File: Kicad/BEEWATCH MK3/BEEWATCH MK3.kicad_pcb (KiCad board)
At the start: 2 copper layers, 40 x 40 mm, 103 parts, among them J1 USB_C_Receptacle_USB2.0, J3 Conn_02x06_Odd_Even, Q1 2N7002, Q2 2N7002, Q3 DMP1045U-7, Q4 BSS138, Q5 BSS138, Q6 BSS138, Q7 BSS138, SW1 TK-074-4, SW2 TK-074-4, U1 ESP32-S3, U3 MPU-6050, U4 MCP73832-2-OT, U5 ME6217C33M5G, U6 LTC3549EDCB#TRMPBF, U7 RYS8830, U8 S-1206B18-M3T1G, Y1 40MHz, Y2 32.768KHz

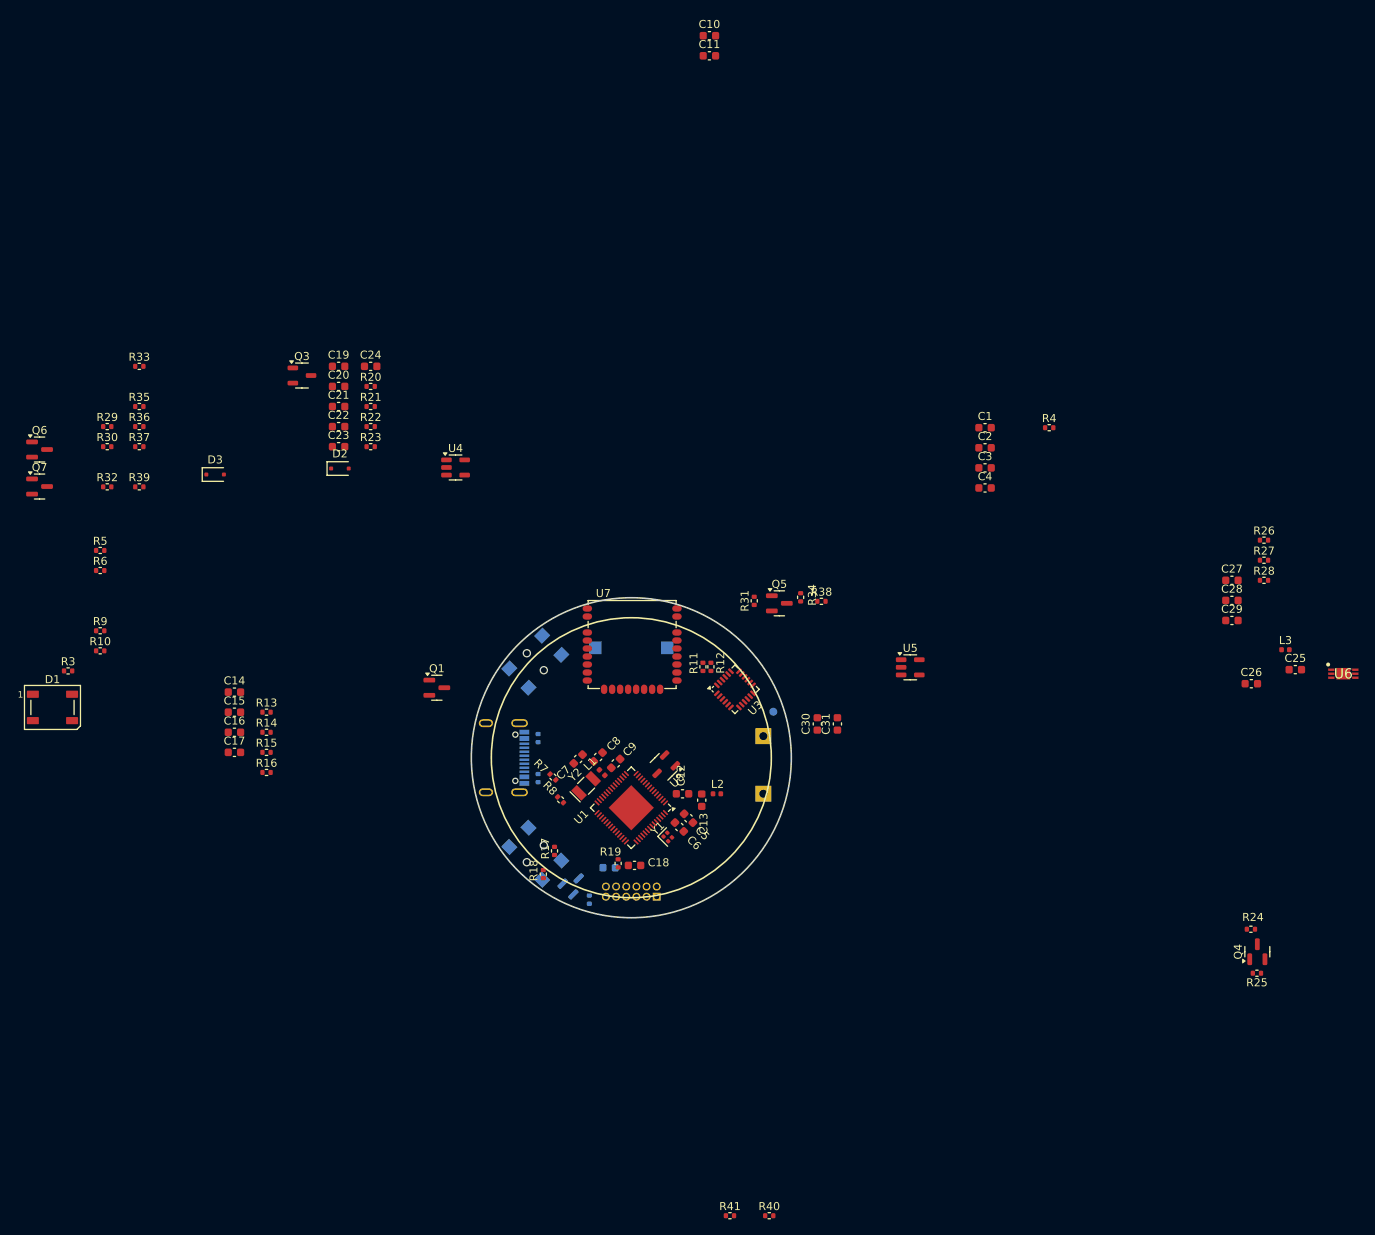
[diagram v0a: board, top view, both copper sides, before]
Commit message: Rough layout placement
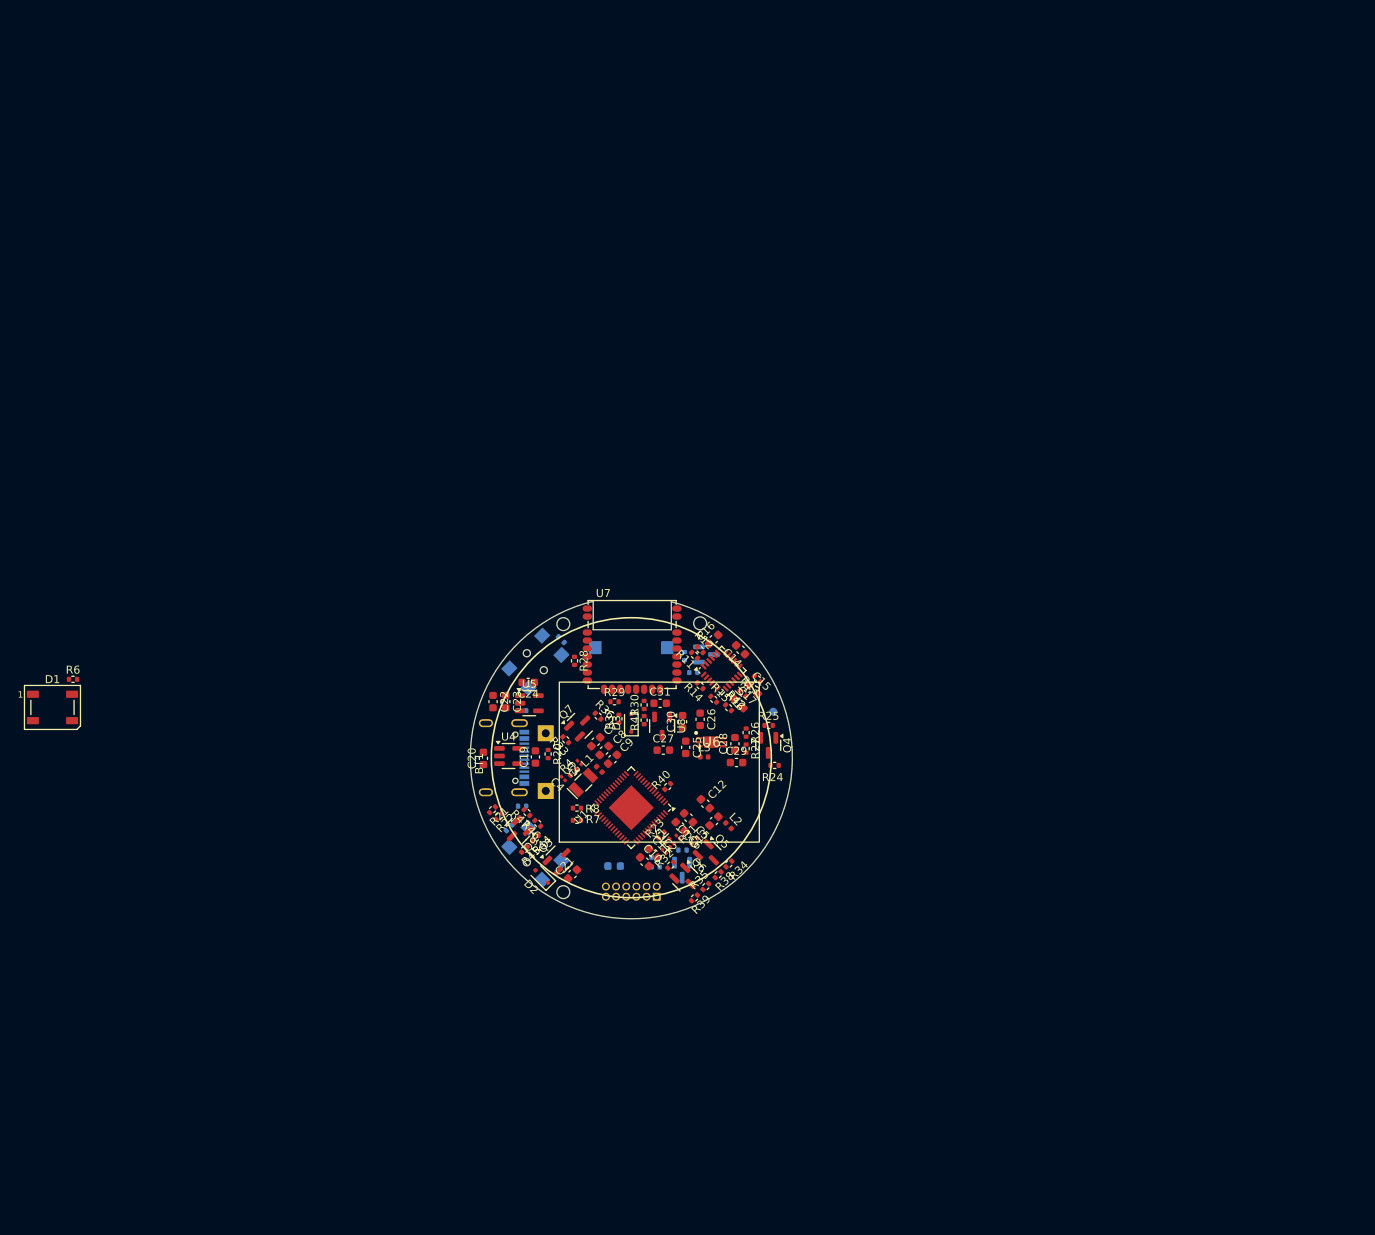
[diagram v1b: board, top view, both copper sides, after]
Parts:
- removed BZ1: BUZZER, Project:CL9032A-CLDZ-SMD Passive Buzzer
- removed the C18 at (150.4, 118.5)
- removed the R19 at (148.3, 118.2)
- added BZ2: Buzzer, Project:CL9032A-CLDZ-SMD Passive Buzzer, B.Cu at (150.0, 91.2)
- added Q9: DMG6968U, Package_TO_SOT_SMD:SOT-23, F.Cu at (135.8, 114.2)
- added R42: 0, Resistor_SMD:R_0402_1005Metric, F.Cu at (163.9, 97.0)
- added R44: 10K, Resistor_SMD:R_0402_1005Metric, F.Cu at (138.0, 115.1)
- added R45: 10K, Resistor_SMD:R_0402_1005Metric, F.Cu at (136.7, 116.5)
- added R46: 100, Resistor_SMD:R_0402_1005Metric, F.Cu at (138.3, 113.2)
- added R47: 10K, Resistor_SMD:R_0402_1005Metric, F.Cu at (136.9, 111.8)
- BT1: moved to F.Cu
- C1, C2, C3, C4: footprint Capacitor_SMD:C_0603_1608Metric -> Capacitor_SMD:C_0201_0603Metric
- Q1: value 2N7002 -> DMG6968U; moved to B.Cu
- Q2: value 2N7002 -> DMG6968U
- R10, R17, R18, R3, R5, R9: moved to B.Cu
- R22: value 22K -> 220
- R23: value 22K -> 5M
- moved C10 103.6 mm to (151.7, 118.0), turned to -45 degrees
- moved C11 99.9 mm to (152.8, 117.0), turned to -45 degrees
- moved Q6 96.9 mm to (156.7, 120.1), turned to -45 degrees
- moved R35 92.8 mm to (159.3, 121.1), turned to 45 degrees
- moved R28 86.8 mm to (142.9, 92.9), turned to -90 degrees
- moved R39 86.4 mm to (157.9, 122.5), turned to -135 degrees
- moved R32 84.8 mm to (154.9, 118.4), turned to 45 degrees
- moved U6 79.5 mm to (160.0, 103.0)
- moved C25 76.8 mm to (156.8, 103.7), turned to -90 degrees
- moved R30 74.5 mm to (151.6, 98.4), turned to 90 degrees
- moved R9 74.3 mm to (157.8, 94.3)
- moved C27 74.2 mm to (154.0, 104.0)
- moved L3 73.9 mm to (159.1, 104.9)
- moved Q7 73.9 mm to (143.6, 101.0), turned to 45 degrees
- moved R4 73.5 mm to (142.8, 106.8), turned to 45 degrees
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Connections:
- C1 pad 1: /ESP32/XTAL_P -> /ESP32/XTAL_N
- C2 pad 1: /ESP32/XTAL_N -> /ESP32/XTAL_P
- D3 pad 2: /RYS8830/GPS_PPS -> /ESP32/GPS_PSS
- J3 pad 1: /Display/TFT_SDI -> /Display/TFT_LEDA
- J3 pad 10: +3.3V -> GND
- J3 pad 11: /Display/TFT_LEDK -> /Display/TFT_D/C
- J3 pad 12: /Display/TFT_RST -> GND
- J3 pad 2: GND -> /Display/TFT_RST
- J3 pad 3: /Display/TFT_SCK -> /Display/TFT_LEDK
- J3 pad 4: GND -> +3.3V
- J3 pad 5: /Display/TFT_CS -> /Display/TFT_SDI
- J3 pad 7: /Display/TFT_D/C -> /Display/TFT_SCK
- J3 pad 9: Net-(J3-Pin_9) -> /Display/TFT_CS
- Q4 pad 3: /RYS8830/GPS_EN -> /ESP32/GPS_EN
- Q7 pad 3: /RYS8830/GPS_RST -> /ESP32/GPS_RST
- R19 pad 1: Net-(J3-Pin_9) -> /Display/TFT_LEDA
- R22 pad 1: VBUS -> Net-(U4-STAT)
- R22 pad 2: /Battery&BMS/PWR_SENSE -> +3.3V
- R23 pad 1: /Battery&BMS/PWR_SENSE -> /ESP32/XTAL_N
- R23 pad 2: GND -> /ESP32/XTAL_P
- R24 pad 1: /RYS8830/GPS_EN -> /ESP32/GPS_EN
- R36 pad 1: /RYS8830/GPS_RST -> /ESP32/GPS_RST
- R37 pad 2: /RYS8830/GPS_PPS -> /ESP32/GPS_PSS
- U1 pad 13: /ESP32/LCD_RST -> /Display/TFT_RST
- U1 pad 14: /ESP32/LCD_DC -> /Display/TFT_D/C
- U1 pad 15: /ESP32/LCD_CS -> /Display/TFT_CS
- U1 pad 16: /ESP32/LCD_MOSI -> /Display/TFT_SDI
- U1 pad 17: /ESP32/LCD_SCK -> /Display/TFT_SCK
- U1 pad 18: /ESP32/MPU_INT -> /ACCELEROMETER/MPU_INT
- U1 pad 27: /ESP32/LED1 -> /Display/TFT_LED_PIN
- U1 pad 38: unconnected-(U1-GPIO33-Pad38) -> /ESP32/LED1
- U1 pad 39: unconnected-(U1-GPIO34-Pad39) -> /Battery&BMS/CHG_ST
- U1 pad 40: unconnected-(U1-GPIO35-Pad40) -> /ESP32/BUZZER_EN
- U1 pad 41: unconnected-(U1-GPIO36-Pad41) -> /Battery&BMS/BAT_SENSE_EN
- U1 pad 7: /ESP32/CHG_ST -> /Battery&BMS/CHG_ST
- U1 pad 8: /ESP32/SDA -> /ACCELEROMETER/MPU_SDA
- U1 pad 9: /ESP32/SCL -> /ACCELEROMETER/MPU_SCL
- U3 pad 9: GND -> Net-(U3-AD0)
- U5 pad 1: /Battery&BMS/PWR_EN -> +VBAT
- Y1 pad 1: /ESP32/XTAL_P -> /ESP32/XTAL_N
- Y1 pad 4: /ESP32/XTAL_N -> /ESP32/XTAL_P
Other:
- board size 40 x 40 mm -> 40.3 x 39.7 mm

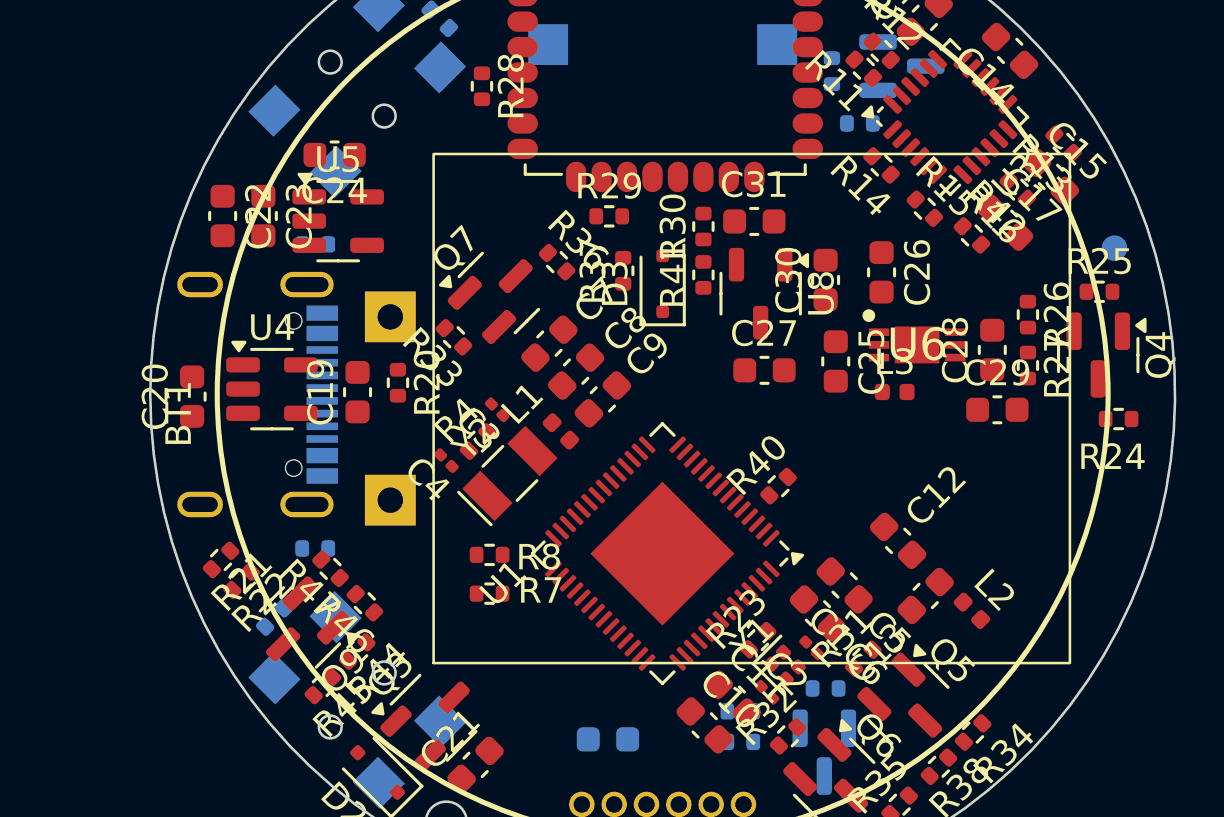
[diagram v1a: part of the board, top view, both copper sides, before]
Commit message: Minor changes in the footprint lib
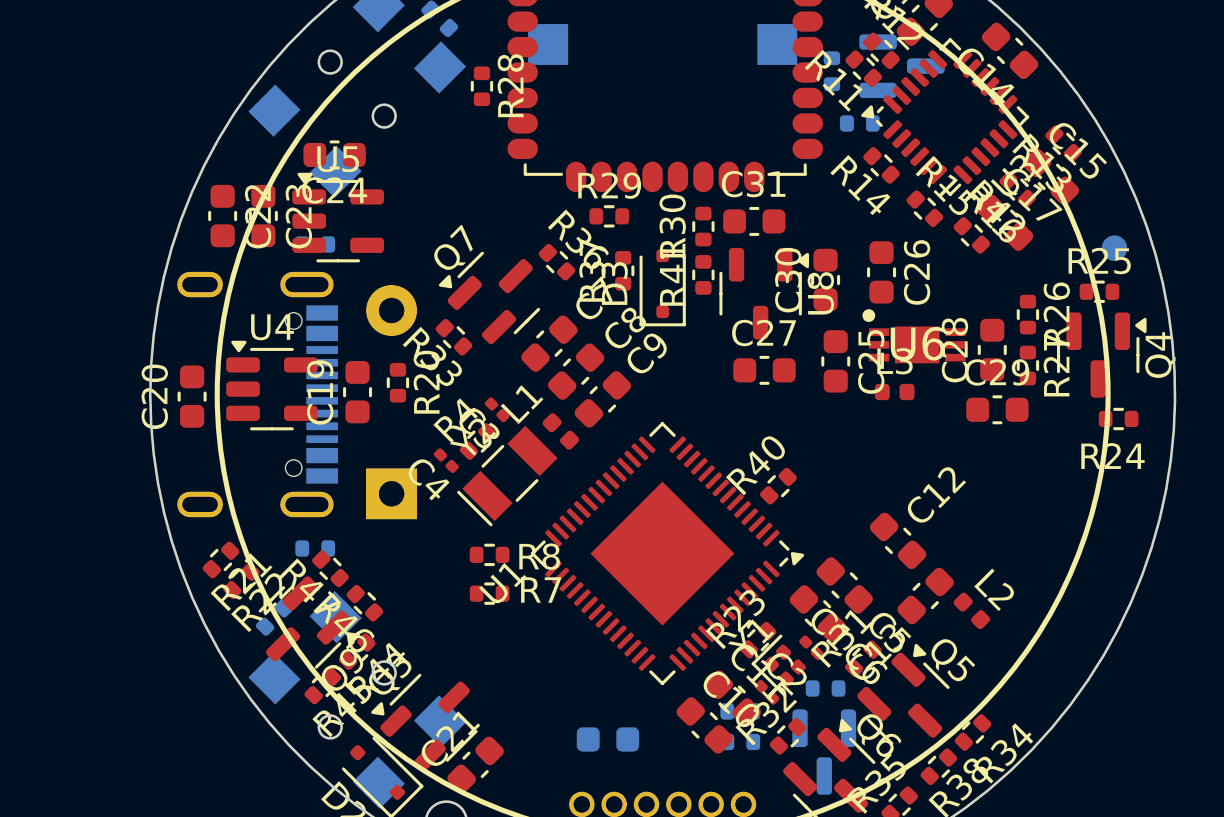
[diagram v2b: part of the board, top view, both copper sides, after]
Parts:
- added meme_2: LOGO, Project:meme_2, B.Cu at (157.8, 105.3)
- BT1: moved to B.Cu
- moved BT1 0.65 mm to (141.2, 105.1), turned to -90 degrees
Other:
- board text added: "Everyone: You can't use PCB for mems Me:"
